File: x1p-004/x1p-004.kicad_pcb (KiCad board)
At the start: 2 copper layers, 20.8 x 28 mm, 21 parts, among them Q1 BC857BS,115, SW1 DSIC01THGET, U1 AD24C02, U2 SN74LVC1T45DBVR, U3 SN74LVC1T45DBVR, U4 SI2301-ZE

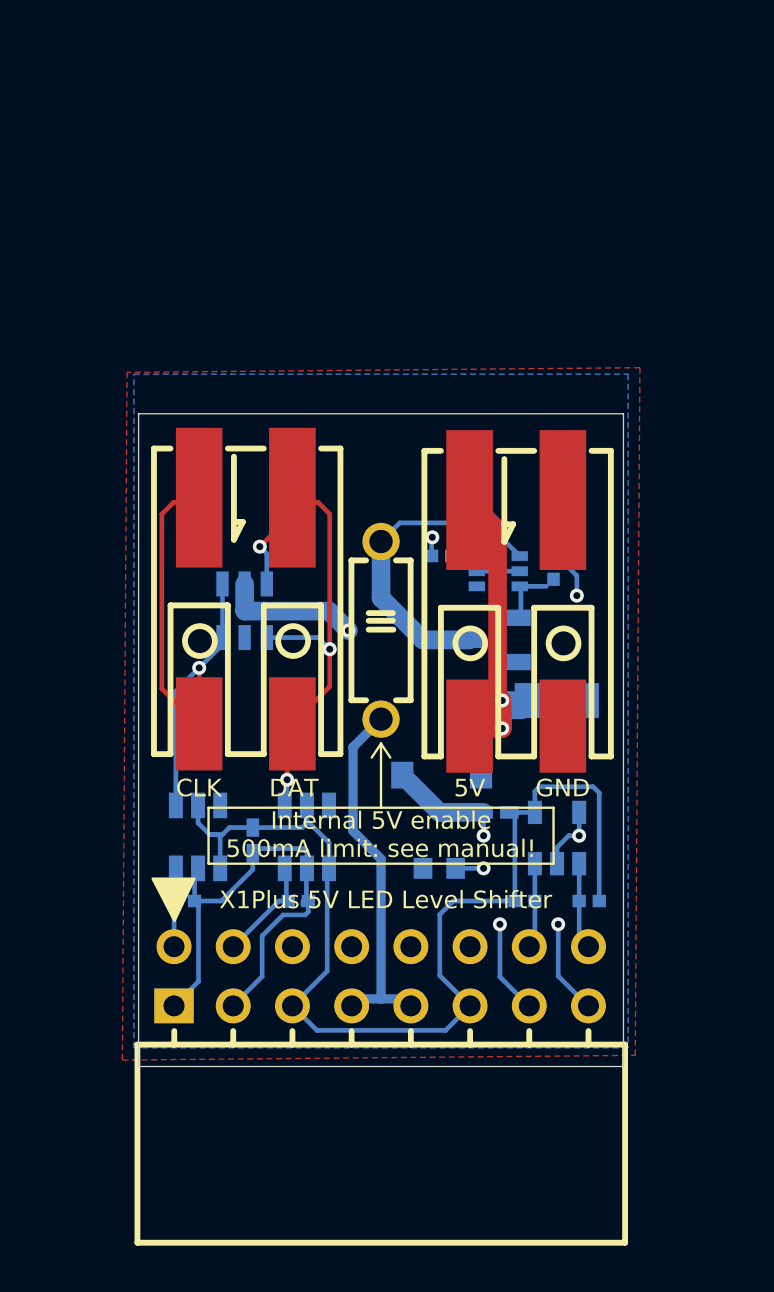
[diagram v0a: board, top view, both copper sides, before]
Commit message: x1p-004: B01 pseudofinal
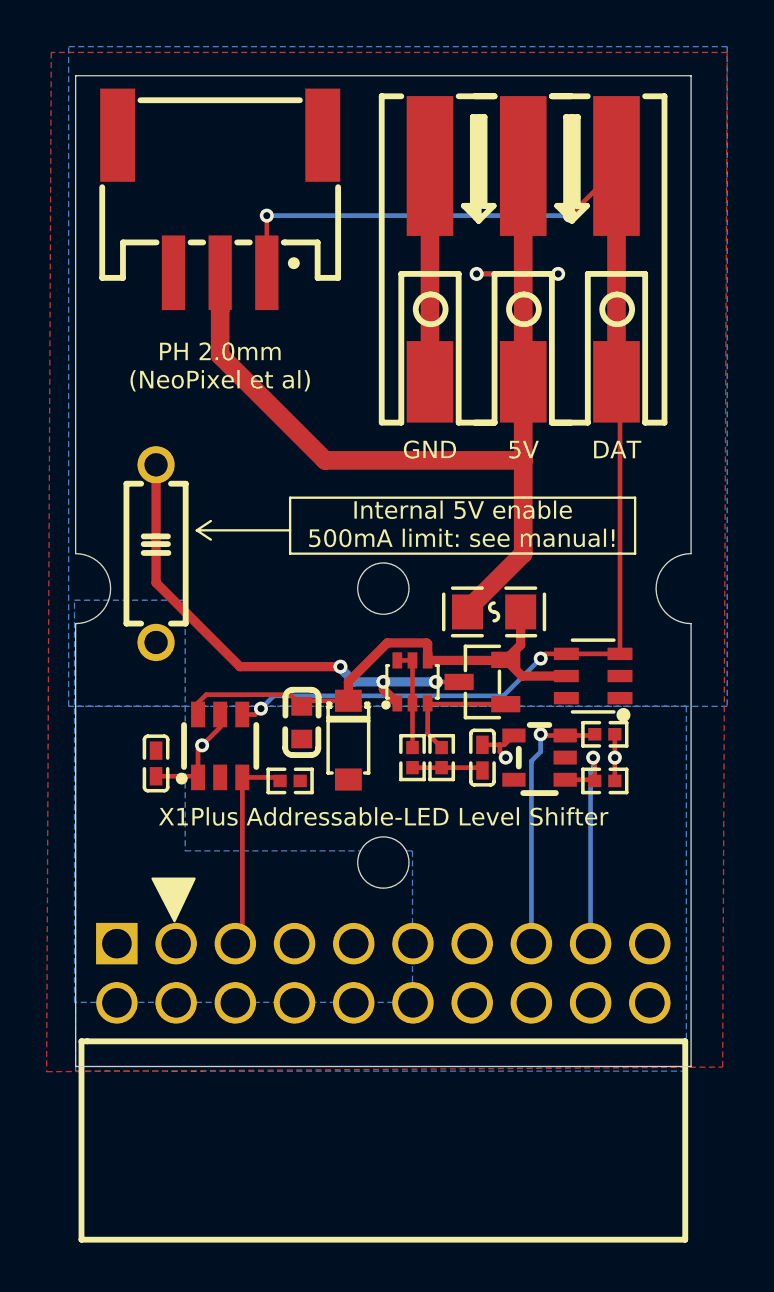
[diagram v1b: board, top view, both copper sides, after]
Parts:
- removed EXT_POWER1, LED1: 2060-452/998-404, x1p-004:CONN-SMD_2060-452
- removed R5: 3.3k, x1p-004:R0402
- added CN1: HC-PH-3AWT, x1p-004:CONN-SMD_3P-P2.0-HC-PH-3AWT, F.Cu at (61.5, 89.5)
- added H1: MountingHole, MountingHole:MountingHole_2.2mm_M2, F.Cu at (68.5, 117.8)
- added H2: MountingHole, MountingHole:MountingHole_2.2mm_M2, F.Cu at (68.5, 106.0)
- C1, C2, C3, D1, D2, F1, Q1, R1, R2, R3, R4, R6, U1, U3, U4: moved to F.Cu
- HDR1: value PM254-2-08-W-8.5 -> 220R-2*10P H=8.5MM Ytype Gold-plated black; footprint x1p-004:HDR-TH_16P-P2.54-H-F-R2-C8-W8.5 -> x1p-004:HDR-TH_20P-P2.54-H-F-R2-C10-S2.54-W10.2
- U2: value SN74LVC1T45DBVR -> 2060-453/998-404; footprint x1p-004:SOT-23-6_L2.9-W1.6-P0.95-LS2.8-BR -> x1p-004:CONN-SMD_2060-453; moved to F.Cu
- moved U2 27.9 mm to (74.5, 92.5)
- moved D2 15.2 mm to (77.5, 109.8), turned to 90 degrees
- moved SW1 10.2 mm to (58.8, 104.5)
- moved R3 9.40 mm to (71.0, 113.2), turned to 90 degrees
- moved R4 8.74 mm to (69.8, 113.2), turned to 90 degrees
- moved C1 8.59 mm to (65.0, 111.8), turned to -90 degrees
- moved R1 7.93 mm to (78.0, 112.2), turned to 0 degrees
- moved Q1 6.01 mm to (69.8, 110.0), turned to 90 degrees
- moved U3 5.39 mm to (61.5, 112.8)
- moved C3 5.30 mm to (58.8, 113.5), turned to 90 degrees
- moved R2 5.19 mm to (78.0, 114.2)
- moved R6 5.16 mm to (64.5, 114.2)
- moved F1 4.66 mm to (73.2, 107.0)
- moved D1 4.27 mm to (67.0, 112.5), turned to -90 degrees
- moved U1 3.53 mm to (75.2, 113.2), turned to 90 degrees
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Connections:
- D2 pad 1: HD0 -> unconnected-(D2-Pad1)
- D2 pad 6: HD0 -> unconnected-(D2-Pad6)
- F1 pad 2: Net-(EXT_POWER1-Pad2) -> Net-(CN1-Pad2)
- HDR1 pad 1: GND -> unconnected-(HDR1-Pad1)
- HDR1 pad 10: unconnected-(HDR1-Pad10) -> 5V
- HDR1 pad 11: 3V3 -> unconnected-(HDR1-Pad11)
- HDR1 pad 12: unconnected-(HDR1-Pad12) -> 5V
- HDR1 pad 13: GND -> unconnected-(HDR1-Pad13)
- HDR1 pad 14: LD6 -> 3V3
- HDR1 pad 15: GND -> LD6
- HDR1 pad 16: LD7 -> GND
- HDR1 pad 2: LD0 -> unconnected-(HDR1-Pad2)
- HDR1 pad 3: GND -> unconnected-(HDR1-Pad3)
- HDR1 pad 4: LD1 -> GND
- HDR1 pad 5: 3V3 -> LD1
- HDR1 pad 6: unconnected-(HDR1-Pad6) -> GND
- HDR1 pad 7: 5V -> unconnected-(HDR1-Pad7)
- HDR1 pad 8: unconnected-(HDR1-Pad8) -> 3V3
- HDR1 pad 9: 5V -> unconnected-(HDR1-Pad9)
- U2 pad 1: 3V3 -> HD1
- U2 pad 2: GND -> Net-(CN1-Pad2)
- U2 pad 3: LD0 -> GND
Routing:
- net Net-(CN1-Pad2): track 0.00 -> 39.6 mm
- net 3V3: track 46.7 -> 9.08 mm, vias 0 -> 3
- net HD1: track 24.7 -> 57.2 mm, vias 3 -> 4
- net GND: track 47.8 -> 17.0 mm, vias 8 -> 2
- net HD0: track 25.7 -> 0.00 mm, vias 1 -> 0
- net 5V_INT: track 0.01 -> 21.8 mm
- net Net-(EXT_POWER1-Pad2): track 17.3 -> 0.00 mm, vias 2 -> 0
- net 5V: track 15.8 -> 0.85 mm
- net LD6: track 3.67 -> 11.9 mm, vias 0 -> 1
- net LD7: track 3.73 -> 10.9 mm, vias 0 -> 1
- net /5V_SW: track 13.9 -> 21.0 mm, vias 0 -> 3
- net LD1: track 5.07 -> 9.20 mm
- net LD0: track 3.51 -> 0.00 mm
- net Net-(U4-G): track 2.45 -> 5.51 mm
- net Net-(Q1-Pad2): track 3.57 -> 4.39 mm
- added copper zone on B.Cu, net 3V3
- added copper zone on B.Cu, net 5V
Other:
- board size 20.8 x 28 mm -> 26.4 x 42.5 mm
- board text added: "PH 2.0mm (NeoPixel et al)"
- board text added: "X1P-004-B01"
- board text added: "X1Plus Addressable-LED Level Shifter"
- board text removed: "CLK"
- board text removed: "X1P-004-A01"
- board text removed: "X1Plus 5V LED Level Shifter"

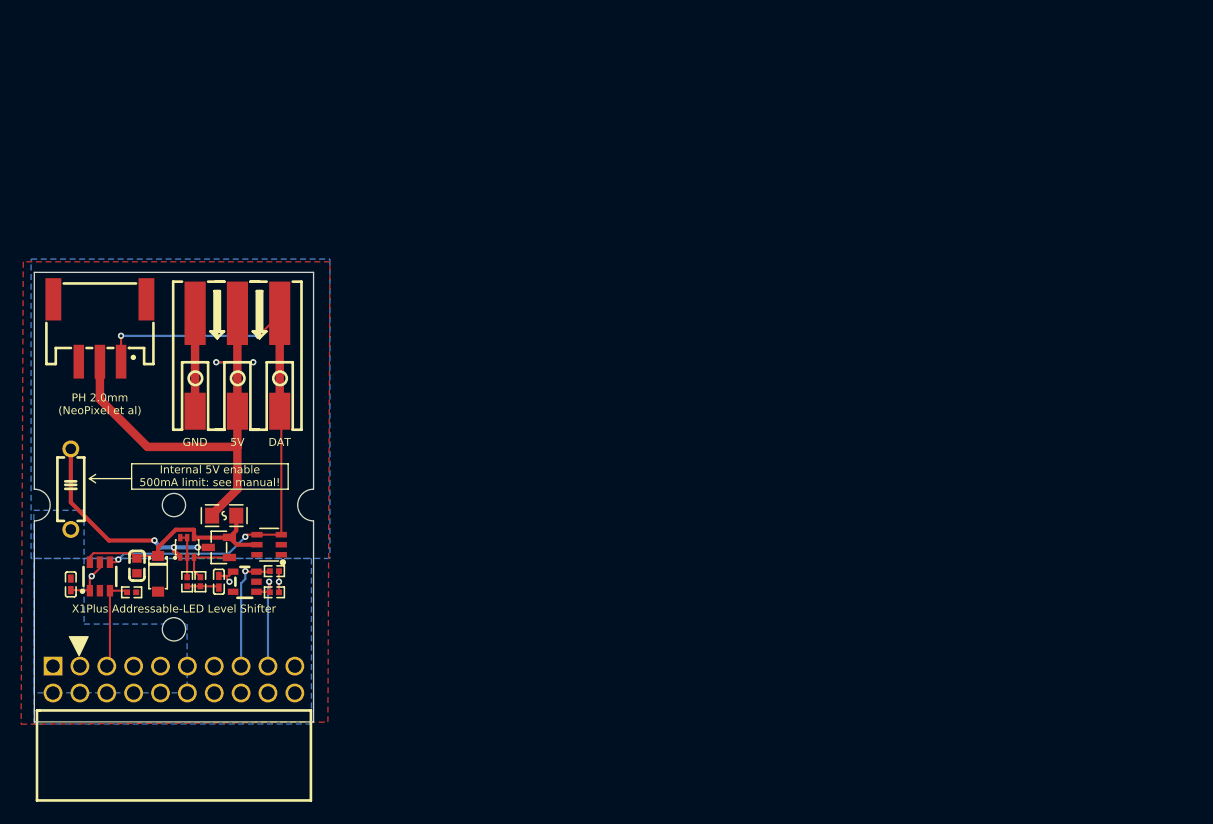
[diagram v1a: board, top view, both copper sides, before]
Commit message: x1p-005: fix up board layout to align with x1p-004
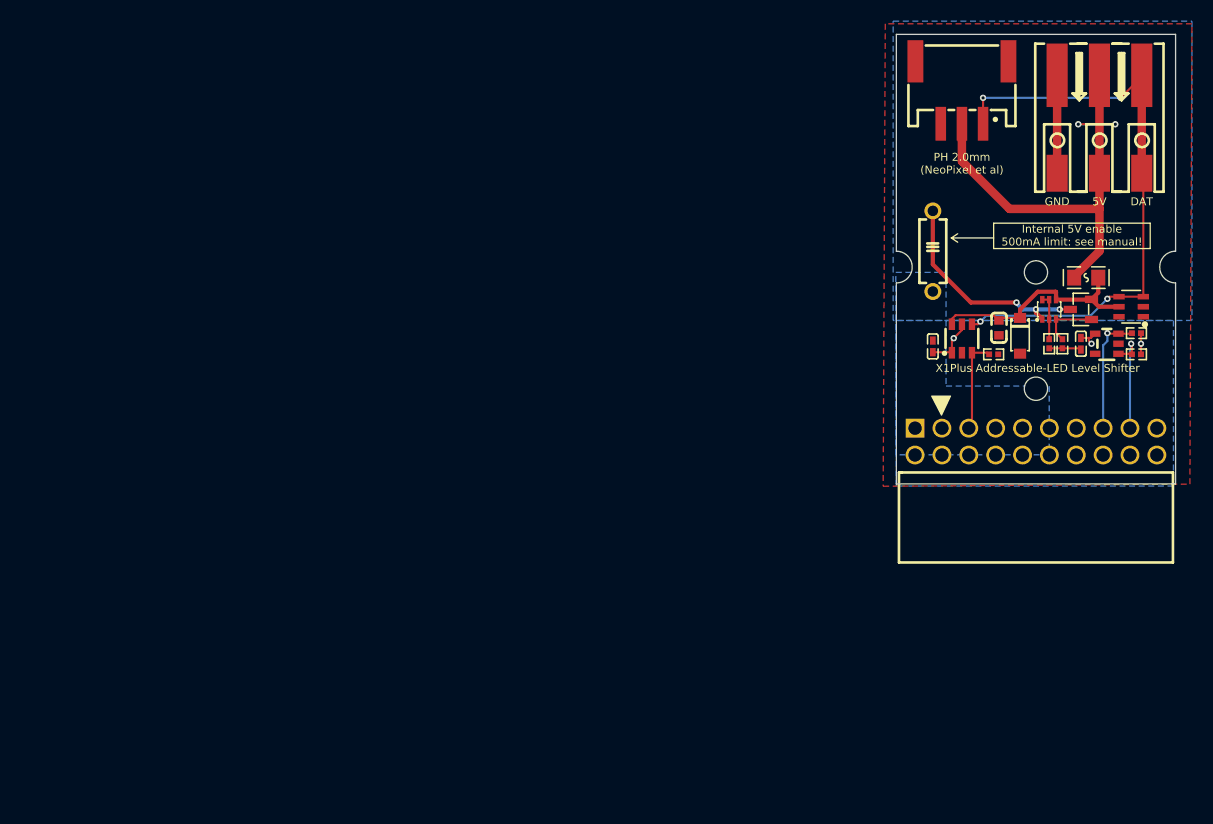
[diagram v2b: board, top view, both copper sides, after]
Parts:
- moved H1 84.6 mm to (150.0, 95.0)
- moved C1 84.5 mm to (146.5, 89.2)
- moved C2 84.5 mm to (154.2, 90.8)
- moved C3 84.5 mm to (140.2, 91.0)
- moved CN1 84.5 mm to (143.0, 67.0)
- moved D1 84.5 mm to (148.5, 90.0)
- moved D2 84.5 mm to (159.0, 87.2)
- moved F1 84.5 mm to (154.8, 84.5)
- moved HDR1 84.5 mm to (150.0, 100.0)
- moved Q1 84.5 mm to (151.2, 87.5)
- moved R1 84.5 mm to (159.5, 89.8)
- moved R2 84.5 mm to (159.5, 91.8)
- moved R3 84.5 mm to (152.5, 90.8)
- moved R4 84.5 mm to (151.2, 90.8)
- moved R6 84.5 mm to (146.0, 91.8)
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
